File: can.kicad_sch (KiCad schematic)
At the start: 19 parts, among them U4 TCAN1044VDRQ1, U5 MCP2518FDT-E/QBB, U6 TCAN1044VDRQ1, Y1 ECS-400-18-33-JGN-TR

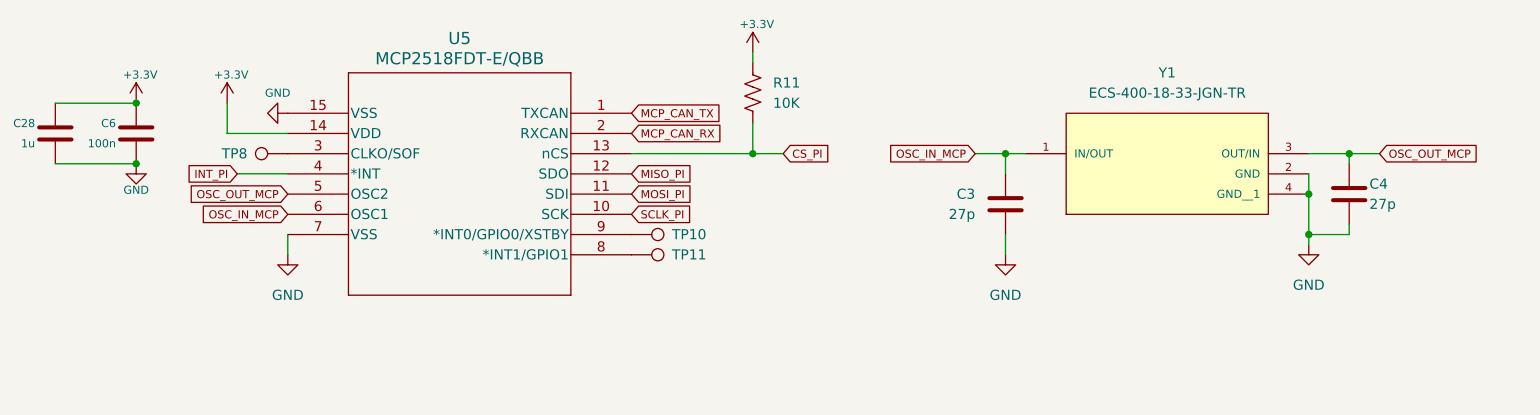
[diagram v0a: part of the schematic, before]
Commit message: Some minor changes
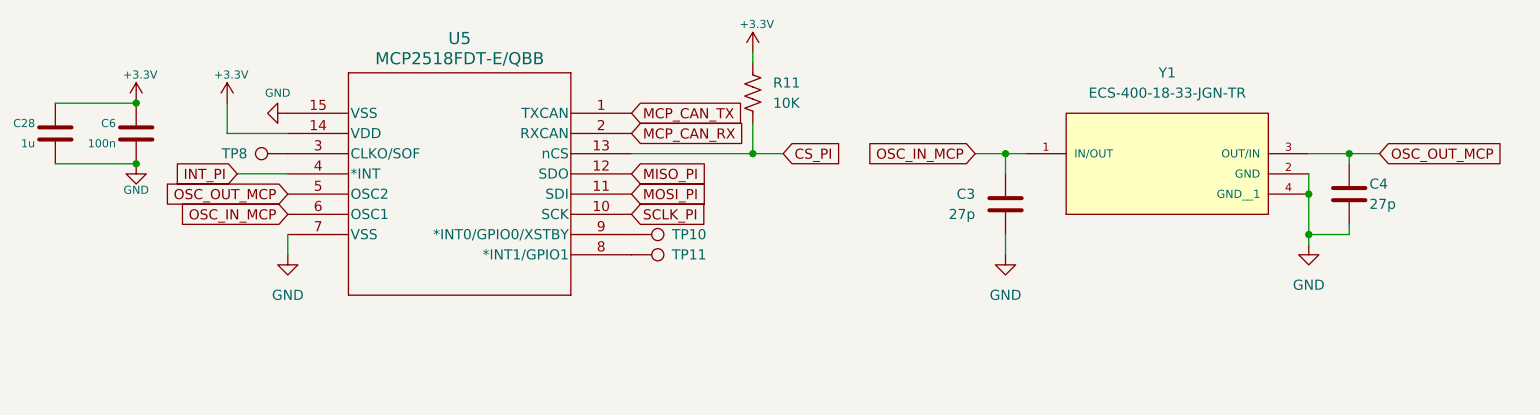
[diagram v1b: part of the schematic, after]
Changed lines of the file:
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@@
 		(effects
 			(font
-				(size 1.016 1.016)
-			)
-			(justify right)
-		)
-		(property "Intersheetrefs" "${INTERSHEET_REFS}"
-			(at 147.5478 40.64 0)
+				(size 1.27 1.27)
+			)
+			(justify right)
+		)
+		(property "Intersheetrefs" "${INTERSHEET_REFS}"
+			(at 144.7471 40.64 0)
 			(hide yes)
 			(show_name no)
@@
 		(effects
 			(font
-				(size 1.016 1.016)
-			)
-			(justify right)
-		)
-		(property "Intersheetrefs" "${INTERSHEET_REFS}"
-			(at 59.5791 43.18 0)
+				(size 1.27 1.27)
+			)
+			(justify right)
+		)
+		(property "Intersheetrefs" "${INTERSHEET_REFS}"
+			(at 57.9637 43.18 0)
 			(hide yes)
 			(show_name no)
@@
 		(effects
 			(font
-				(size 1.016 1.016)
-			)
-			(justify left)
-		)
-		(property "Intersheetrefs" "${INTERSHEET_REFS}"
-			(at 222.1069 40.64 0)
+				(size 1.27 1.27)
+			)
+			(justify left)
+		)
+		(property "Intersheetrefs" "${INTERSHEET_REFS}"
+			(at 225.2462 40.64 0)
 			(hide yes)
 			(show_name no)
@@
 		(effects
 			(font
-				(size 1.016 1.016)
-			)
-			(justify right)
-		)
-		(property "Intersheetrefs" "${INTERSHEET_REFS}"
-			(at 61.1878 48.26 0)
+				(size 1.27 1.27)
+			)
+			(justify right)
+		)
+		(property "Intersheetrefs" "${INTERSHEET_REFS}"
+			(at 58.3871 48.26 0)
 			(hide yes)
 			(show_name no)
@@
 		(effects
 			(font
-				(size 1.016 1.016)
-			)
-			(justify left)
-		)
-		(property "Intersheetrefs" "${INTERSHEET_REFS}"
-			(at 123.3855 45.72 0)
+				(size 1.27 1.27)
+			)
+			(justify left)
+		)
+		(property "Intersheetrefs" "${INTERSHEET_REFS}"
+			(at 125.3396 45.72 0)
 			(hide yes)
 			(show_name no)
@@
 		(effects
 			(font
-				(size 1.016 1.016)
-			)
-			(justify left)
-		)
-		(property "Intersheetrefs" "${INTERSHEET_REFS}"
-			(at 127.1109 38.1 0)
+				(size 1.27 1.27)
+			)
+			(justify left)
+		)
+		(property "Intersheetrefs" "${INTERSHEET_REFS}"
+			(at 129.9962 38.1 0)
 			(hide yes)
 			(show_name no)
@@
 		(effects
 			(font
-				(size 1.016 1.016)
-			)
-			(justify left)
-		)
-		(property "Intersheetrefs" "${INTERSHEET_REFS}"
-			(at 126.869 35.56 0)
+				(size 1.27 1.27)
+			)
+			(justify left)
+		)
+		(property "Intersheetrefs" "${INTERSHEET_REFS}"
+			(at 129.6938 35.56 0)
 			(hide yes)
 			(show_name no)
@@
 		(effects
 			(font
-				(size 1.016 1.016)
-			)
-			(justify left)
-		)
-		(property "Intersheetrefs" "${INTERSHEET_REFS}"
-			(at 140.7422 40.64 0)
+				(size 1.27 1.27)
+			)
+			(justify left)
+		)
+		(property "Intersheetrefs" "${INTERSHEET_REFS}"
+			(at 142.2729 40.64 0)
 			(hide yes)
 			(show_name no)
@@
 		(effects
 			(font
-				(size 1.016 1.016)
-			)
-			(justify left)
-		)
-		(property "Intersheetrefs" "${INTERSHEET_REFS}"
-			(at 123.3855 43.18 0)
+				(size 1.27 1.27)
+			)
+			(justify left)
+		)
+		(property "Intersheetrefs" "${INTERSHEET_REFS}"
+			(at 125.3396 43.18 0)
 			(hide yes)
 			(show_name no)
@@
 		(effects
 			(font
-				(size 1.016 1.016)
-			)
-			(justify left)
-		)
-		(property "Intersheetrefs" "${INTERSHEET_REFS}"
-			(at 123.5307 48.26 0)
+				(size 1.27 1.27)
+			)
+			(justify left)
+		)
+		(property "Intersheetrefs" "${INTERSHEET_REFS}"
+			(at 125.521 48.26 0)
 			(hide yes)
 			(show_name no)
@@
 		(effects
 			(font
-				(size 1.016 1.016)
-			)
-			(justify right)
-		)
-		(property "Intersheetrefs" "${INTERSHEET_REFS}"
-			(at 59.8331 45.72 0)
-			(hide yes)
-			(show_name no)
+				(size 1.27 1.27)
+			)
+			(justify right)
+		)
+		(property "Intersheetrefs" "${INTERSHEET_REFS}"
+			(at 56.6938 45.72 0)
+			(hide yes)
+			(show_name no)

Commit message: updated footprints
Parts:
- U4, U6: footprint D0008A-IPC_A -> (none)
- U5: footprint VDFN14_QBB_MCH -> (none)
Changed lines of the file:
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@@
 			)
 		)
-		(property "Footprint" "D0008A-IPC_A"
+		(property "Footprint" ""
 			(at 111.76 130.81 0)
 			(hide yes)
@@
 			)
 		)
-		(property "Footprint" "VDFN14_QBB_MCH"
+		(property "Footprint" ""
 			(at 72.39 35.56 0)
 			(hide yes)
@@
 			)
 		)
-		(property "Footprint" "D0008A-IPC_A"
+		(property "Footprint" ""
 			(at 111.76 86.36 0)
 			(hide yes)

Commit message: added footprints
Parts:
- C12, C13, C17, C28, C3, C4, C6, C7, C8: footprint (none) -> Capacitor_SMD:C_0603_1608Metric_Pad1.08x0.95mm_HandSolder
- R11, R12, R13: footprint (none) -> Resistor_SMD:R_0603_1608Metric_Pad0.98x0.95mm_HandSolder
- TP10, TP11, TP8: footprint (none) -> TestPoint:TestPoint_Pad_D1.5mm
- U5: footprint (none) -> rov_MCP_footprint:VDFN14_QBB_MCH-M

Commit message: almost done with footprints
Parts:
- U4, U6: footprint (none) -> rov_TCAN_footprint:D0008A-IPC_A
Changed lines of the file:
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@@
 			)
 		)
-		(property "Footprint" ""
+		(property "Footprint" "rov_TCAN_footprint:D0008A-IPC_A"
 			(at 111.76 130.81 0)
 			(hide yes)
@@
 			)
 		)
-		(property "Footprint" ""
+		(property "Footprint" "rov_TCAN_footprint:D0008A-IPC_A"
 			(at 111.76 86.36 0)
 			(hide yes)
